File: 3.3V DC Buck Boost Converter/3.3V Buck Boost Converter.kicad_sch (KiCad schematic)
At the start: 5 parts

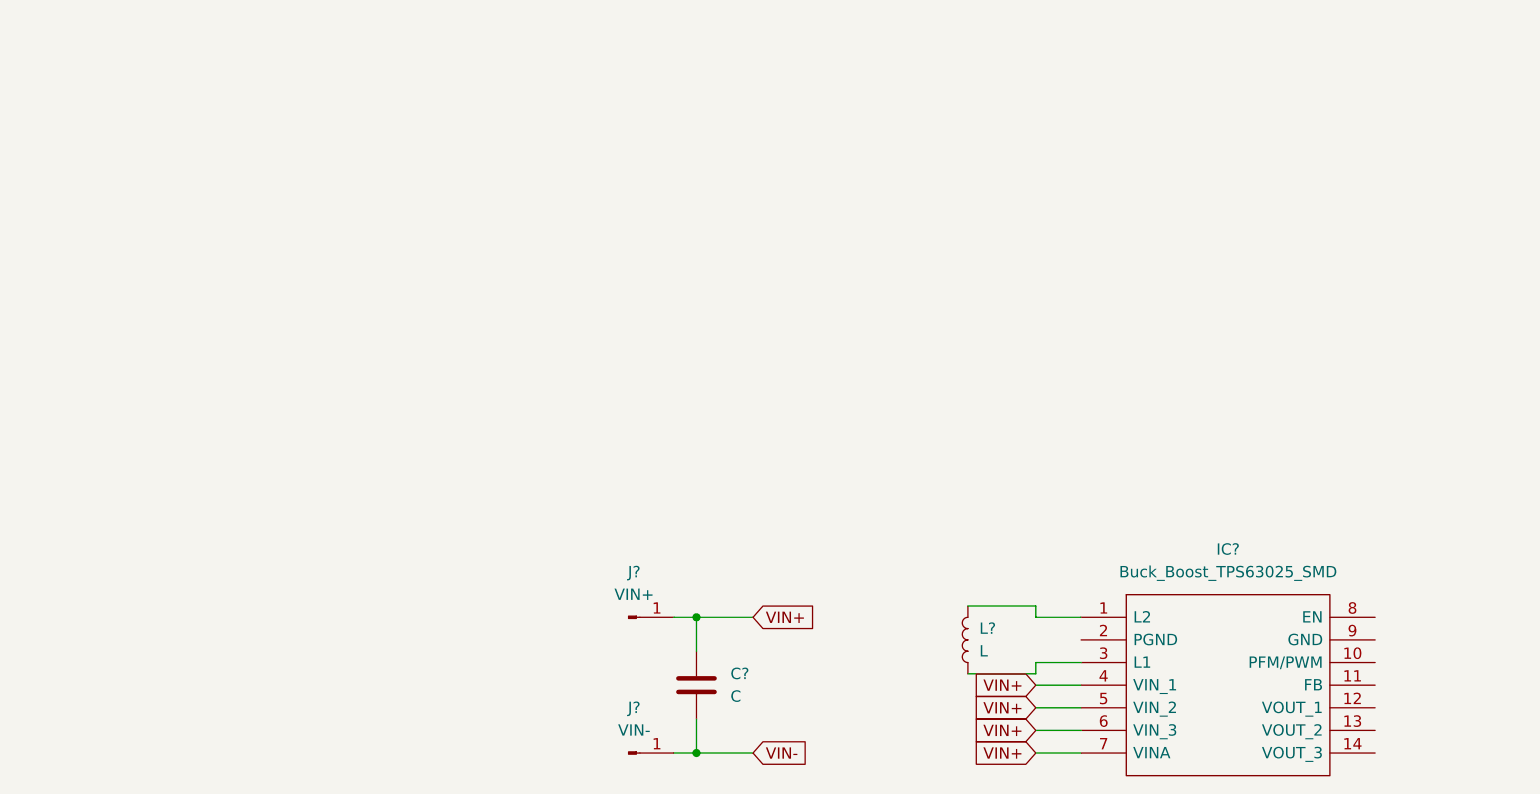
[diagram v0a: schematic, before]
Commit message: updates
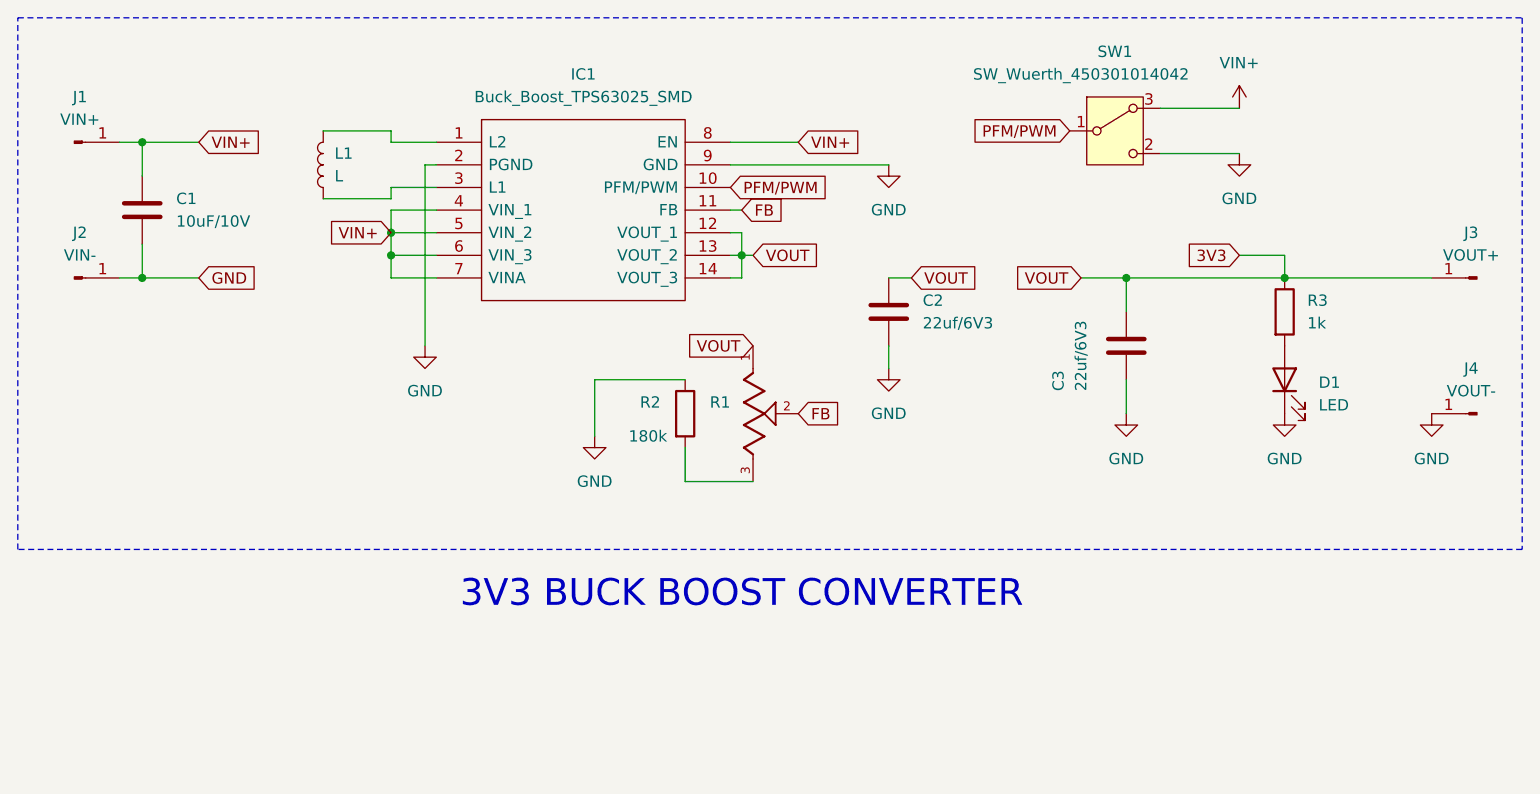
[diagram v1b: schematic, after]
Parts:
- added C2, C3: 22uf/6V3, Capacitor_THT:C_Radial_D6.3mm_H11.0mm_P2.50mm, symbol Device:C
- added D1: LED, LED_THT:LED_D3.0mm, symbol Device:LED
- added J3: VOUT+, Library:TestPoint_Pad_1.0x1.0mm, symbol Connector:Conn_01x01_Pin
- added J4: VOUT-, Library:TestPoint_Pad_1.0x1.0mm, symbol Connector:Conn_01x01_Pin
- added R1: PT01-D120K1-B103, Library:TrimPot_10k_SMD, symbol New_Library_0:PT01-D120K1-B103
- added R2: 180k, Resistor_THT:R_Axial_DIN0207_L6.3mm_D2.5mm_P10.16mm_Horizontal, symbol Device:R
- added R3: 1k, Resistor_THT:R_Axial_DIN0207_L6.3mm_D2.5mm_P10.16mm_Horizontal, symbol Device:R
- added SW1: SW_Wuerth_450301014042, Button_Switch_THT:SW_Slide-03_Wuerth-WS-SLTV_10x2.5x6.4_P2.54mm, symbol Switch:SW_Wuerth_450301014042
- C1: renamed from C?; value C -> 10uF/10V; footprint (none) -> Capacitor_THT:C_Radial_D6.3mm_H11.0mm_P2.50mm
- IC1: renamed from IC?; footprint TPS630250RNCT -> Library:IC_BuckBoost_TPS630250RNCT_VQFN14_2x3mm
- J1, J2: renamed from J?; footprint (none) -> Library:TestPoint_Pad_1.0x1.0mm
- L1: renamed from L?; footprint (none) -> SymScs_Ft:XFL7015102MEB
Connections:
- net VIN- is gone; now on net GND: C1.2, J2.1 (Pin_1)
- net VIN+: now also IC1.8 (EN), SW1.3 (A)
- net PFM/PWM: now reaches IC1.10 (PFM/PWM)
- net PFM/PWM: now also SW1.1 (B)
- net FB: now reaches IC1.11 (FB)
- net FB: now also R1.2
- net 3V3: now reaches IC1.12 (VOUT_1)
- net 3V3: now also IC1.13 (VOUT_2), IC1.14 (VOUT_3), C2.1, C3.1, J3.1 (Pin_1), R1.1, R3.1
- net GND: now reaches IC1.2 (PGND)
- net GND: now also IC1.9 (GND), C2.2, C3.2, D1.1 (K), J4.1 (Pin_1), R2.1, SW1.2 (C)
- new net: R1.3, R2.2
- new net: D1.2 (A), R3.2
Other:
- note added: "3V3 BUCK BOOST CONVERTER"
- moved on the sheet: C1, IC1, J1, J2, L1
